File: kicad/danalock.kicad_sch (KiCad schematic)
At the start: 11 parts, among them J1 Conn_02x02_Top_Bottom, J2 Conn_01x02, J3 Conn_01x03, U1 ESP32mini, U2 DSN-MINI-360, U3 DRV8871DDA

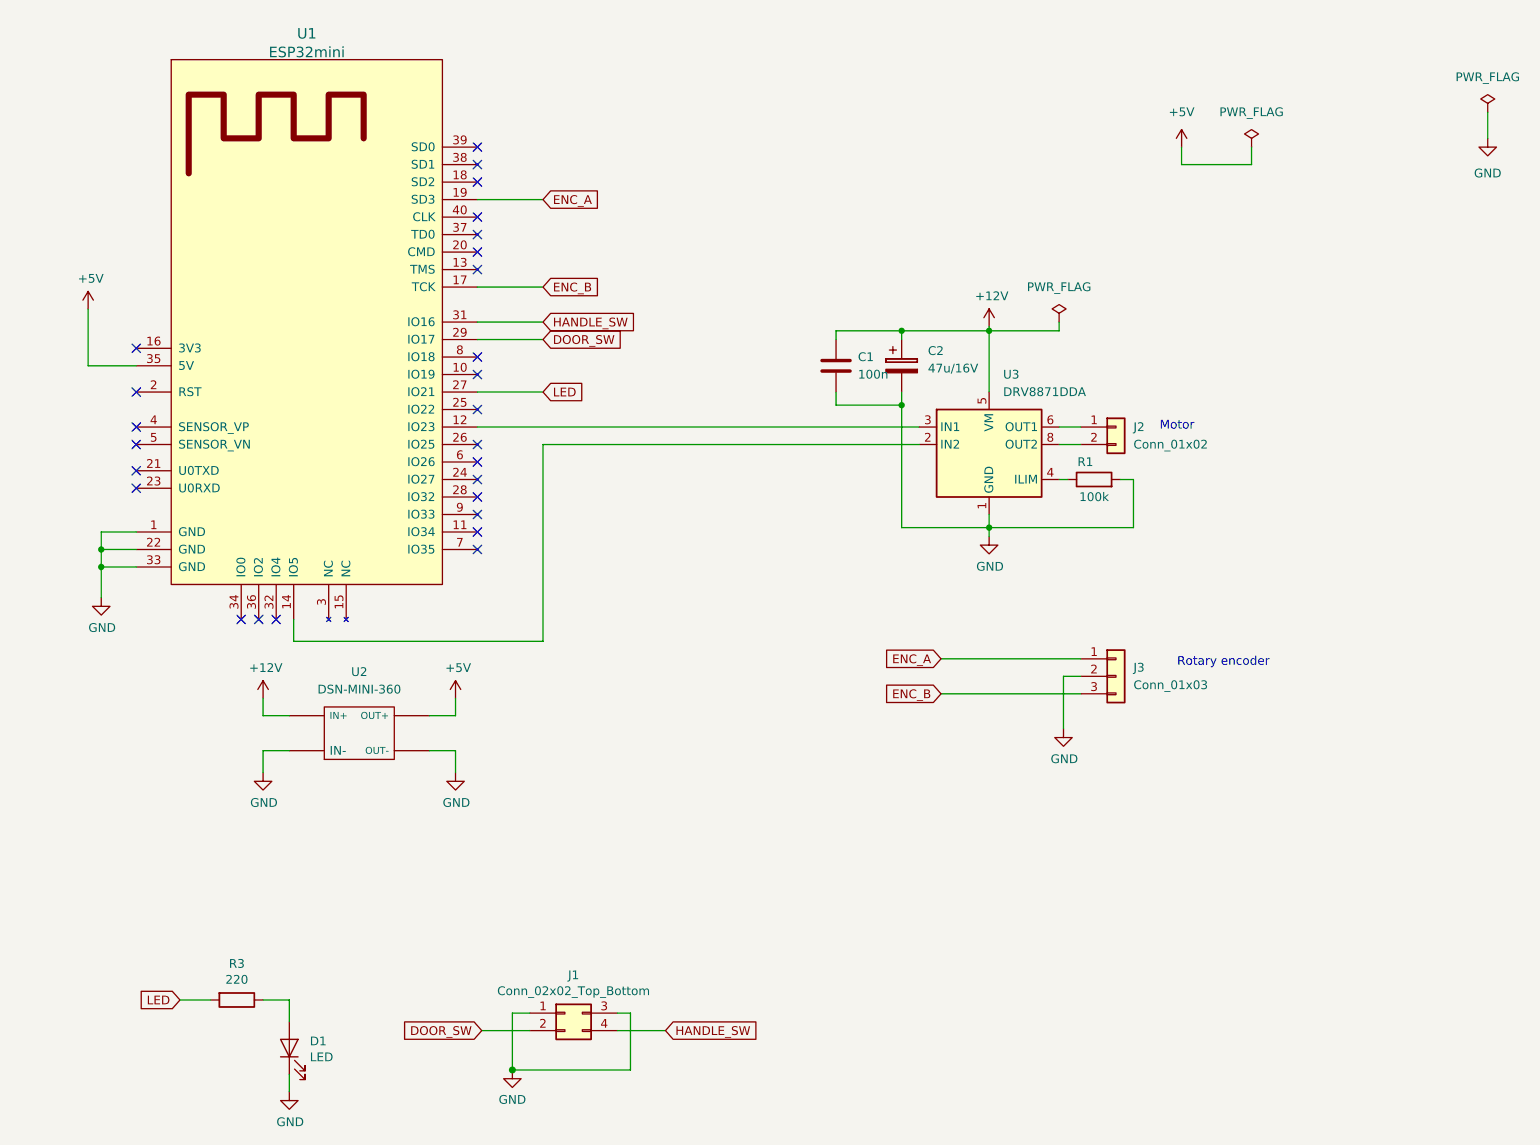
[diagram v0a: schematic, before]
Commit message: KiCAD update.
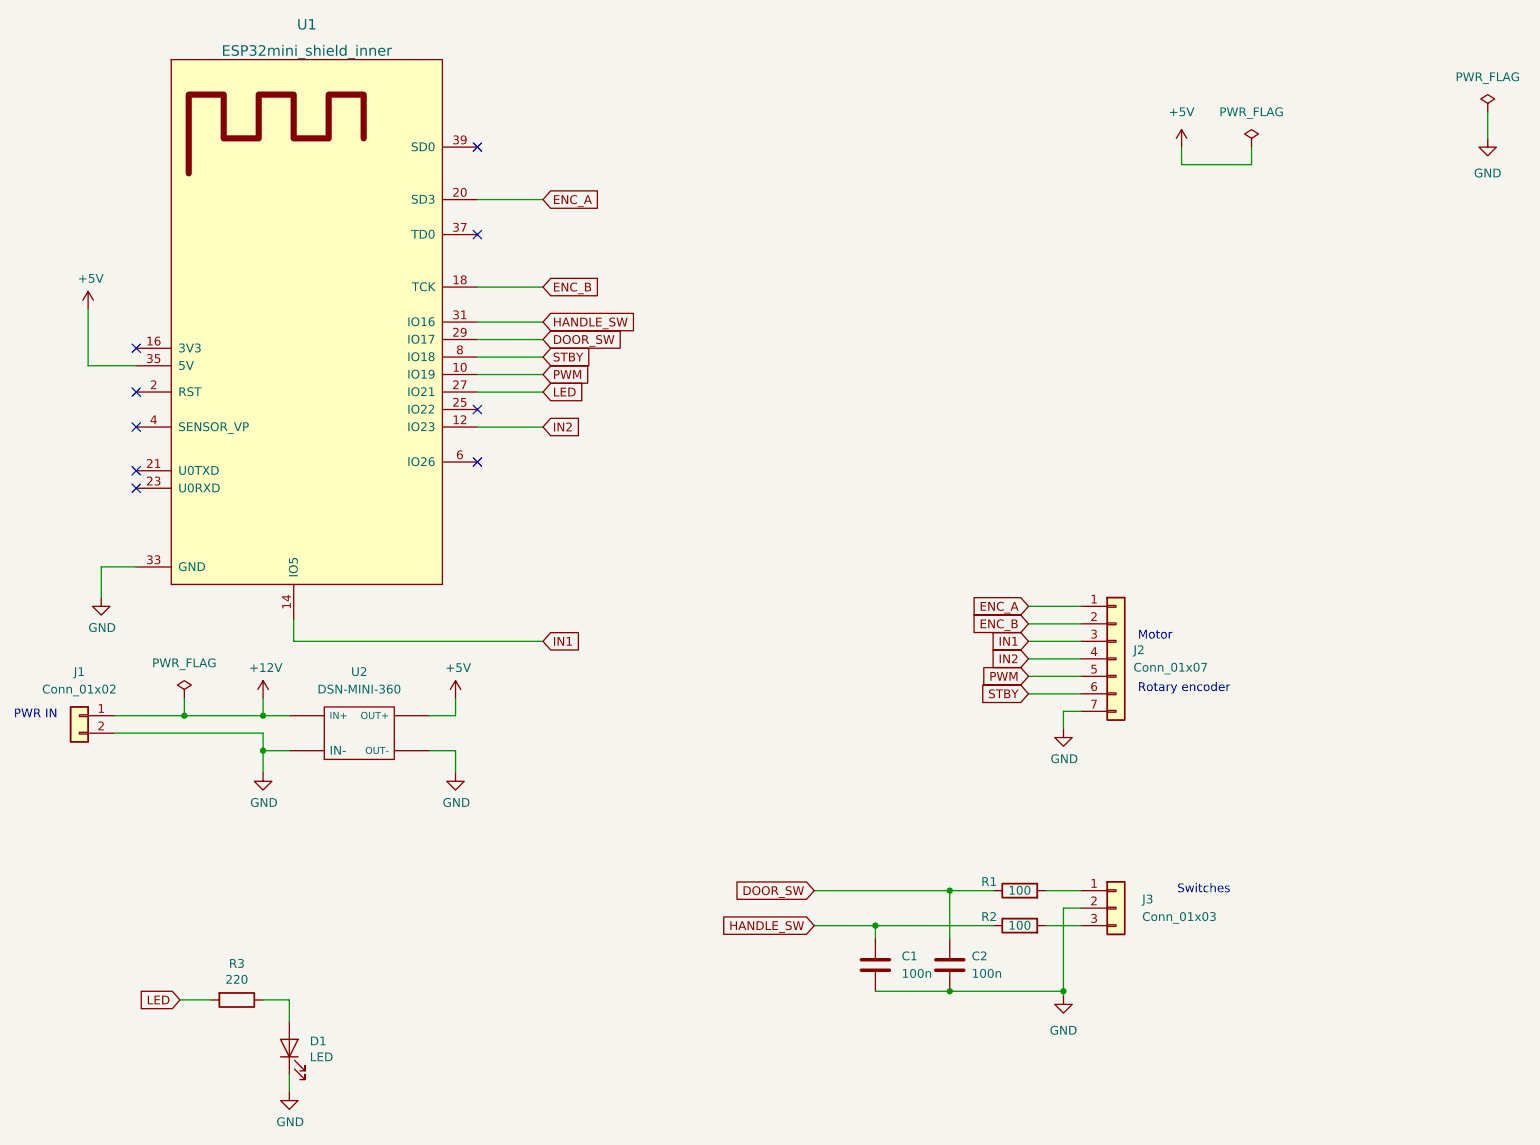
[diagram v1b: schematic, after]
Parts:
- removed C2: 47u/16V, symbol Device:CP
- removed J1: Conn_02x02_Top_Bottom, symbol Connector_Generic:Conn_02x02_Top_Bottom
- removed J2: Conn_01x02, symbol Connector_Generic:Conn_01x02
- removed U1: ESP32mini, ESP32mini:ESP32mini, symbol esp32mini:ESP32mini
- removed U3: DRV8871DDA, Package_SO:Texas_HTSOP-8-1EP_3.9x4.9mm_P1.27mm_EP2.95x4.9mm_Mask2.4x3.1mm_ThermalVias, symbol Driver_Motor:DRV8871DDA
- added C2: 100n, Capacitor_SMD:C_0603_1608Metric, symbol Device:C
- added J1: Conn_01x02, Connector_JST:JST_XH_B2B-XH-A_1x02_P2.50mm_Vertical, symbol Connector_Generic:Conn_01x02
- added J2: Conn_01x07, Connector_PinSocket_2.00mm:PinSocket_1x07_P2.00mm_Vertical, symbol Connector_Generic:Conn_01x07
- added R2: 100, Resistor_SMD:R_0603_1608Metric, symbol Device:R
- added U1: ESP32mini_shield_inner, hal9k:ESP32mini_shield_inner, symbol esp32mini-shield-inner:ESP32mini_shield_inner
- C1: footprint (none) -> Capacitor_SMD:C_0603_1608Metric
- D1: footprint (none) -> LED_THT:LED_D5.0mm
- J3: footprint (none) -> Connector_PinSocket_2.00mm:PinSocket_1x03_P2.00mm_Vertical
- R1: value 100k -> 100; footprint (none) -> Resistor_SMD:R_0603_1608Metric
- R3: footprint (none) -> Resistor_SMD:R_0603_1608Metric
- U2: footprint (none) -> hal9k:DSN-MINI-360
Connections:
- net +12V: now also J1.1 (Pin_1); no longer C1.1
- net +5V: now also U1.35 (5V)
- net DOOR_SW: now also R1.1, C2.1, U1.29 (IO17)
- net ENC_A: now also J2.1 (Pin_1), U1.20 (SD3); no longer J3.1 (Pin_1)
- net ENC_B: now also J2.2 (Pin_2), U1.18 (TCK); no longer J3.3 (Pin_3)
- net GND: now also C2.2, J1.2 (Pin_2), J2.7 (Pin_7), U1.33 (GND); no longer R1.2
- net HANDLE_SW: now also C1.1, R2.1, U1.31 (IO16)
- net LED: now also U1.27 (IO21)
- new net: J3.1 (Pin_1), R1.2
- new net: J3.3 (Pin_3), R2.2
- new net IN1: J2.3 (Pin_3), U1.14 (IO5)
- new net IN2: J2.4 (Pin_4), U1.12 (IO23)
- new net PWM: J2.5 (Pin_5), U1.10 (IO19)
- new net STBY: J2.6 (Pin_6), U1.8 (IO18)
- no-connect marks 26 -> 9
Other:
- note added: "PWR IN"
- note added: "Switches"
